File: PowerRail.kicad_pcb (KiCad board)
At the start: 4 copper layers, 43.2 x 43.2 mm, 65 parts, among them P10 LEDS, P11 CONN_01X06, P12 CONN_01X02, P13 USB_OTG, P14 CONN_01X06, P15 JTI-PWR, P9 ADJ, U5 TPS65530, U6 VEC2616

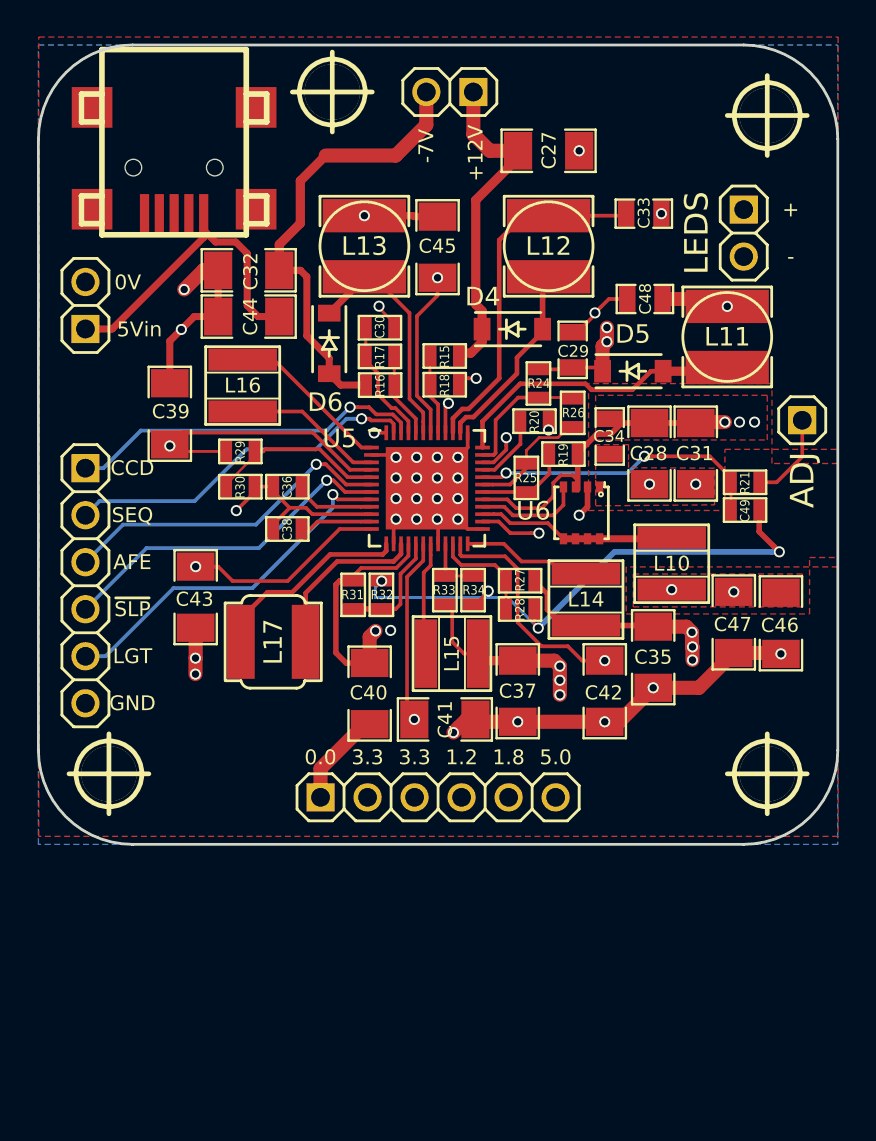
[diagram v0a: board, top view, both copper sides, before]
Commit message: More work
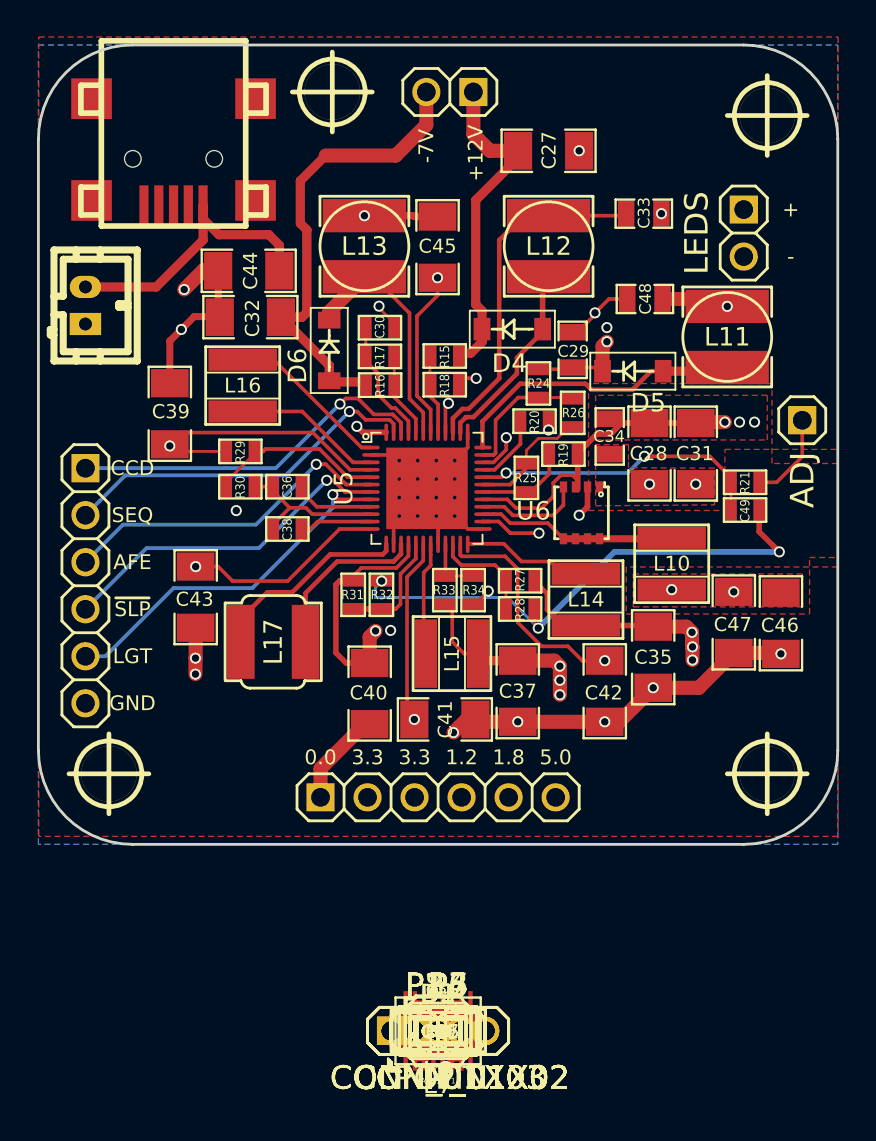
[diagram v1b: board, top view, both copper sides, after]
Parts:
- added C1, C2, C8, C9: 2.2uF, smd:SM0603, F.Cu at (154.6, 124.8)
- added C10, C15: 4.7uF, smd:SM0603, F.Cu at (154.6, 124.8)
- added C11: 6.8pF, smd:SM0603, F.Cu at (154.6, 124.8)
- added C12: 33pF, smd:SM0603, F.Cu at (154.6, 124.8)
- added C13: 10uF, smd:SM0603, F.Cu at (154.6, 124.8)
- added C14: 220pF, smd:SM0603, F.Cu at (154.6, 124.8)
- added C16: 3.9nF, smd:SM0603, F.Cu at (154.6, 124.8)
- added C17: 22.0uF, smd:SM1206, F.Cu at (154.6, 124.8)
- added C18: 12pF, smd:SM0603, F.Cu at (154.6, 124.8)
- added C19: 8.2nF, smd:SM0603, F.Cu at (154.6, 124.8)
- added C20: 68pF, smd:SM0603, F.Cu at (154.6, 124.8)
- added C21, C22, C6: 1.0uF, smd:SM0603, F.Cu at (154.6, 124.8)
- added C23, C54: 4.7uF, smd:SM0805, F.Cu at (154.6, 124.8)
- added C24: 1.0uF, smd:SM0805, F.Cu at (154.6, 124.8)
- added C25, C26: 10.0uF, smd:SM1206, F.Cu at (154.6, 124.8)
- added C3: 4.7pF, smd:SM0603, F.Cu at (154.6, 124.8)
- added C4, C5, C53, C55: 0.1uF, smd:SM0603, F.Cu at (154.6, 124.8)
- added C50: 2.2uF, smd:SM0805, F.Cu at (154.6, 124.8)
- added C51: 22uF, smd:SM1206, F.Cu at (154.6, 124.8)
- added C52: 47pF, smd:SM0603, F.Cu at (154.6, 124.8)
- added C7: 10pF, smd:SM0603, F.Cu at (154.6, 124.8)
- added D1: D_Schottky, engstad:diode-smd-powerdi-123, F.Cu at (154.6, 124.8)
- added D2, D3: DFLS240, engstad:diode-smd-powerdi-123, F.Cu at (154.6, 124.8)
- added L4: 10 uH, engstad:inductor-smd-1212, F.Cu at (154.6, 124.8)
- added L6: 2.2uH, engstad:inductor-smd-1210, F.Cu at (154.6, 124.8)
- added L7: 3.3uH, engstad:inductor-smd-1212-lqh3np, F.Cu at (154.6, 124.8)
- added L8: 0.47uH, engstad:inductor-smd-1210, F.Cu at (154.6, 124.8)
- added L9: 1.0uH, engstad:inductor-smd-1210, F.Cu at (154.6, 124.8)
- added P1, P2: CONN_01X03, xess:HDR_1x3, F.Cu at (154.6, 124.8)
- added P3, P4, P5, P6: CONN_01X02, xess:HDR_1x2, F.Cu at (154.6, 124.8)
- added P7: PIN, xess:HDR_1x2, F.Cu at (154.6, 124.8)
- added P8: POUT, xess:HDR_1x3, F.Cu at (154.6, 124.8)
- added R1: 430k, smd:SM0603, F.Cu at (154.6, 124.8)
- added R10: 6.98k, smd:SM0603, F.Cu at (154.6, 124.8)
- added R11: 66.5k, smd:SM0603, F.Cu at (154.6, 124.8)
- added R12: 68.1k, smd:SM0603, F.Cu at (154.6, 124.8)
- added R13: 3.09 Ohm, smd:SM0603, F.Cu at (154.6, 124.8)
- added R14: 6.19 Ohm, smd:SM0603, F.Cu at (154.6, 124.8)
- added R2: 280k, smd:SM0603, F.Cu at (154.6, 124.8)
- added R22: 324k, smd:SM0603, F.Cu at (154.6, 124.8)
- added R23: 549k, smd:SM0603, F.Cu at (154.6, 124.8)
- added R3: 562k, smd:SM0603, F.Cu at (154.6, 124.8)
- added R35: 18.7k, smd:SM0603, F.Cu at (154.6, 124.8)
- added R36: 56.2k, smd:SM0603, F.Cu at (154.6, 124.8)
- added R4: 100k, smd:SM0603, F.Cu at (154.6, 124.8)
- added R5: 118k, smd:SM0603, F.Cu at (154.6, 124.8)
- added R6: 13.3k, smd:SM0603, F.Cu at (154.6, 124.8)
- added R7: 21.5k, smd:SM0603, F.Cu at (154.6, 124.8)
- added R8: 5.23k, smd:SM0603, F.Cu at (154.6, 124.8)
- added R9: 4.75k, smd:SM0603, F.Cu at (154.6, 124.8)
- added T1, T2: NET-TIE, engstad:net-tie-0.5mm, F.Cu at (154.6, 124.8)
- added U1: LT3472, w_smd_qfn:dfn10-3x3, F.Cu at (154.6, 124.8)
- added U2: LMR62014, w_smd_trans:sot23-5, F.Cu at (154.6, 124.8)
- added U3: LM3674, w_smd_trans:sot23-5, F.Cu at (154.6, 124.8)
- added U4: ADP5071, w_smd_qfn:pvqfn-n20, F.Cu at (154.6, 124.8)
- D4, D5, D6: footprint Diodes_SMD:SOD-123 -> engstad:diode-sod-123
- P13: footprint w_conn_pc:conn_usb_B_mini_smd -> engstad:conn-smd-usb-b-mini
- P15: footprint xess:HDR_1x2 -> w_conn_jst-ph:b2b-ph-kl
- U5: footprint Housings_DFN_QFN:UQFN-48-1EP_6x6mm_Pitch0.4mm -> engstad:qfn-48-p
- moved C32 2.53 mm to (144.4, 86.2)
- moved C44 2.47 mm to (144.4, 83.7)
- moved P13 0.47 mm to (140.3, 76.3)
- moved D6 0.38 mm to (148.7, 88.0)
- turned U5 to 270 degrees
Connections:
- P15 pad 1: /TPS65530/VBATT -> GND
- P15 pad 2: GND -> /TPS65530/VBATT
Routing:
- net /TPS65530/VBATT: track 160.5 -> 167.3 mm
- net GND: track 50.8 -> 47.9 mm, vias 7 -> 6
- net /TPS65530/VOUT_CCD-: track 24.8 -> 25.8 mm
- net GNDPWR: vias 32 -> 16
- net (no net): vias 0 -> 1
- added copper zone on B.Cu, net GNDPWR
- removed copper zone on B.Cu, net GND
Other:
- rule trace_min: 0.127 -> 0.1524
- board text removed: "0V"
- board text removed: "5Vin"
